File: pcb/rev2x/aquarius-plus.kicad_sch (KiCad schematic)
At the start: 179 parts, among them J1 Cassette in, J10 Audio out, J11 Hand controller 2, J12 ESP USB Host, J13 Power in, J14 FPGA spare, J15 Expansion port, J16 ESP32 spare, J2 Cassette out, J3 Amphenol GSD090012SEU, J4 Printer, J5 Hand controller 1, J6 VGA, J7 DBG, Q1 BC847C, Q2 BC847C, SW1 SW_DPDT_x2, U1 XC3S200-4TQG144, U10 IS61C5128AS-25QLI, U13 SST39SF020A-55-4C-WHE, U14 74LVC4245APW, U15 LDL1117S33R, U16 MCP1700T-2502E/TT, U17 LD1117S12, U2 SN74CBTD3861PWR, U3 MAX3221ECPWR, U4 SN74CBTD3861PWR, U5 ESP32-S2-SOLO-N4R2, U6 SN74CBTD3861PWR, U7 Z84C0010AEG, U8 SN74CBTD3861PWR, X1 ECS-5032MV-143-CN-TR

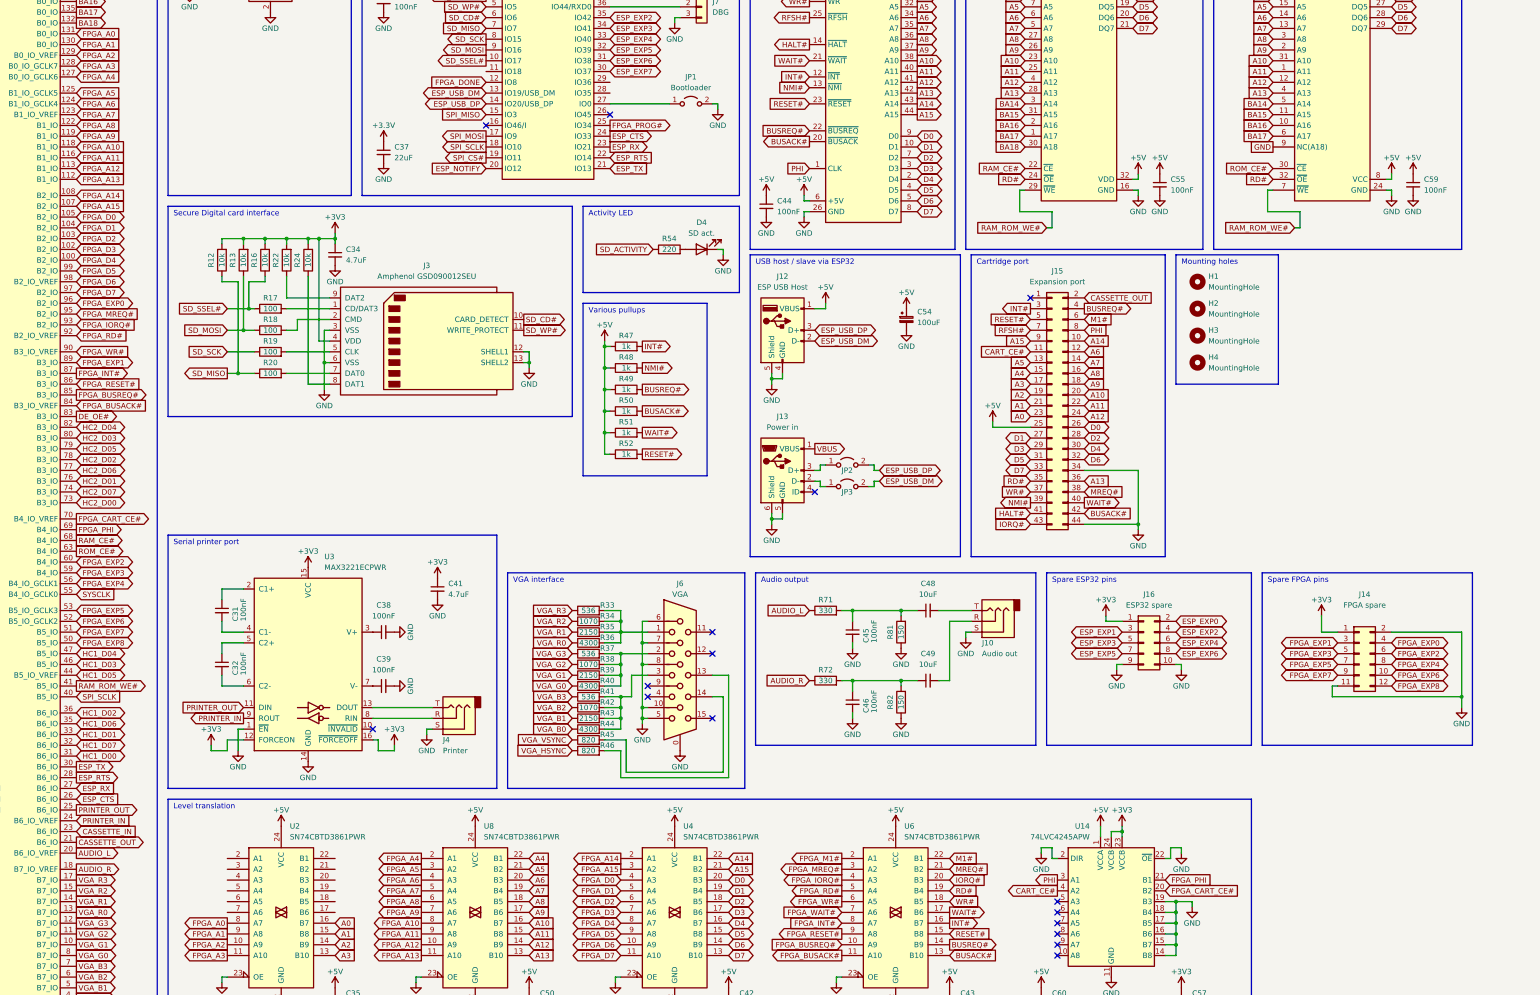
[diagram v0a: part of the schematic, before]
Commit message: PCB rev2x Corrections
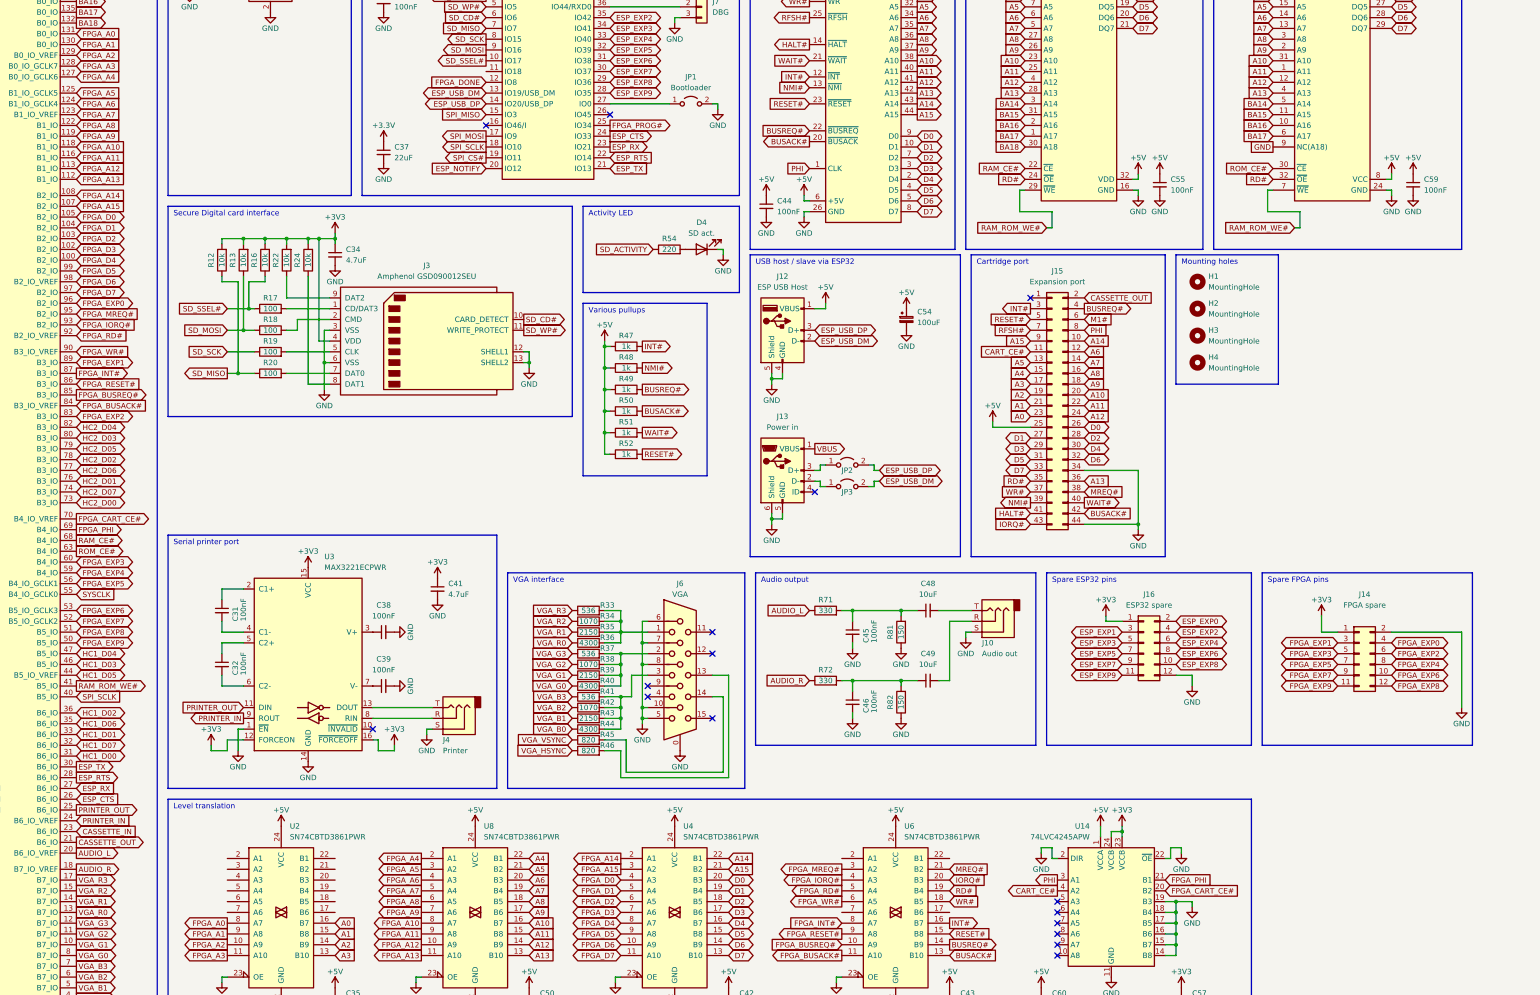
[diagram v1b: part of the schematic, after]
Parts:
- J16: footprint Connector_PinHeader_2.54mm:PinHeader_2x05_P2.54mm_Vertical -> Connector_PinHeader_2.54mm:PinHeader_2x06_P2.54mm_Vertical; symbol Connector_Generic:Conn_02x05_Odd_Even -> Connector_Generic:Conn_02x06_Odd_Even
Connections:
- net DE_OE# is gone; now on net FPGA_EXP2: U1.83 (B3_IO)
- net ESP_EXP7: now also J16.9 (Pin_9)
- net FPGA_EXP2: no longer U1.60 (B4_IO)
- net FPGA_EXP3: now also U1.60 (B4_IO); no longer U1.59 (B4_IO)
- net FPGA_EXP4: now also U1.59 (B4_IO); no longer U1.56 (B4_IO_GCLK1)
- net FPGA_EXP5: now also U1.56 (B4_IO_GCLK1); no longer U1.53 (B5_IO_GCLK3)
- net FPGA_EXP6: now also U1.53 (B5_IO_GCLK3); no longer U1.52 (B5_IO_GCLK2)
- net FPGA_EXP7: now also U1.52 (B5_IO_GCLK2); no longer U1.51 (B5_IO)
- net FPGA_EXP8: now also U1.51 (B5_IO); no longer U1.50 (B5_IO)
- net GND: now also J16.12 (Pin_12); no longer J14.11 (Pin_11), J16.10 (Pin_10), J16.9 (Pin_9)
- net M1#: no longer U6.22 (B1)
- net WAIT#: no longer U6.17 (B6)
- net ESP_EXP9: now reaches U5.28 (IO35)
- net ESP_EXP9: now also J16.11 (Pin_11)
- net ESP_EXP8: now reaches U5.29 (IO36)
- net ESP_EXP8: now also J16.10 (Pin_10)
- net FPGA_M1#: no longer names the net of U6.2 (A1)
- net FPGA_WAIT#: no longer names the net of U6.7 (A6)
- new net FPGA_EXP9: J14.11 (Pin_11), U1.50 (B5_IO)
